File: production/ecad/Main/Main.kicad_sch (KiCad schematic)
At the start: 1 part, among them J1 61204021621

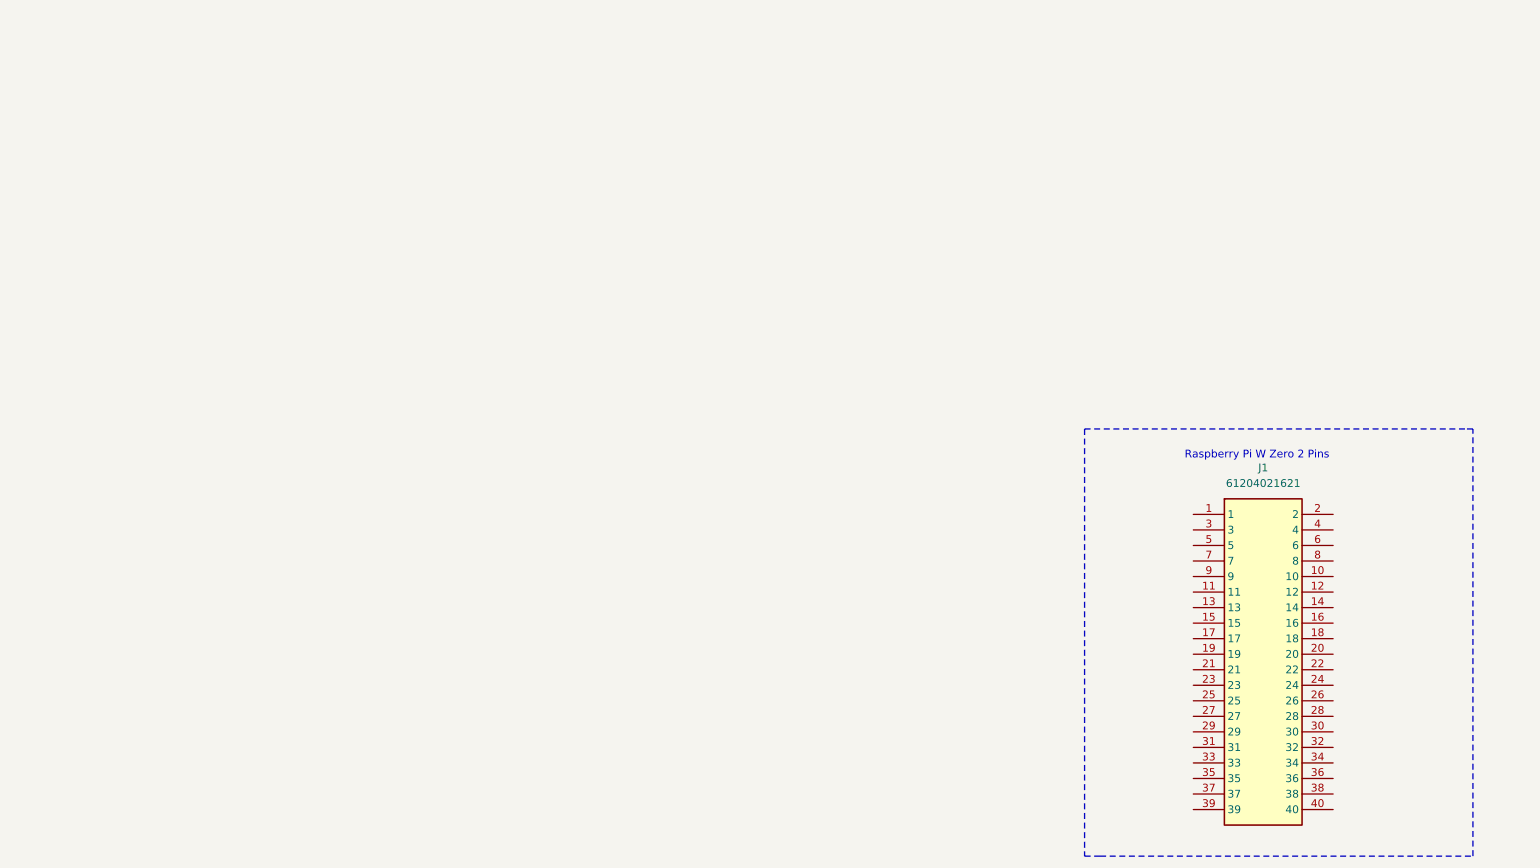
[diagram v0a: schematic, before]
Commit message: touches to schem
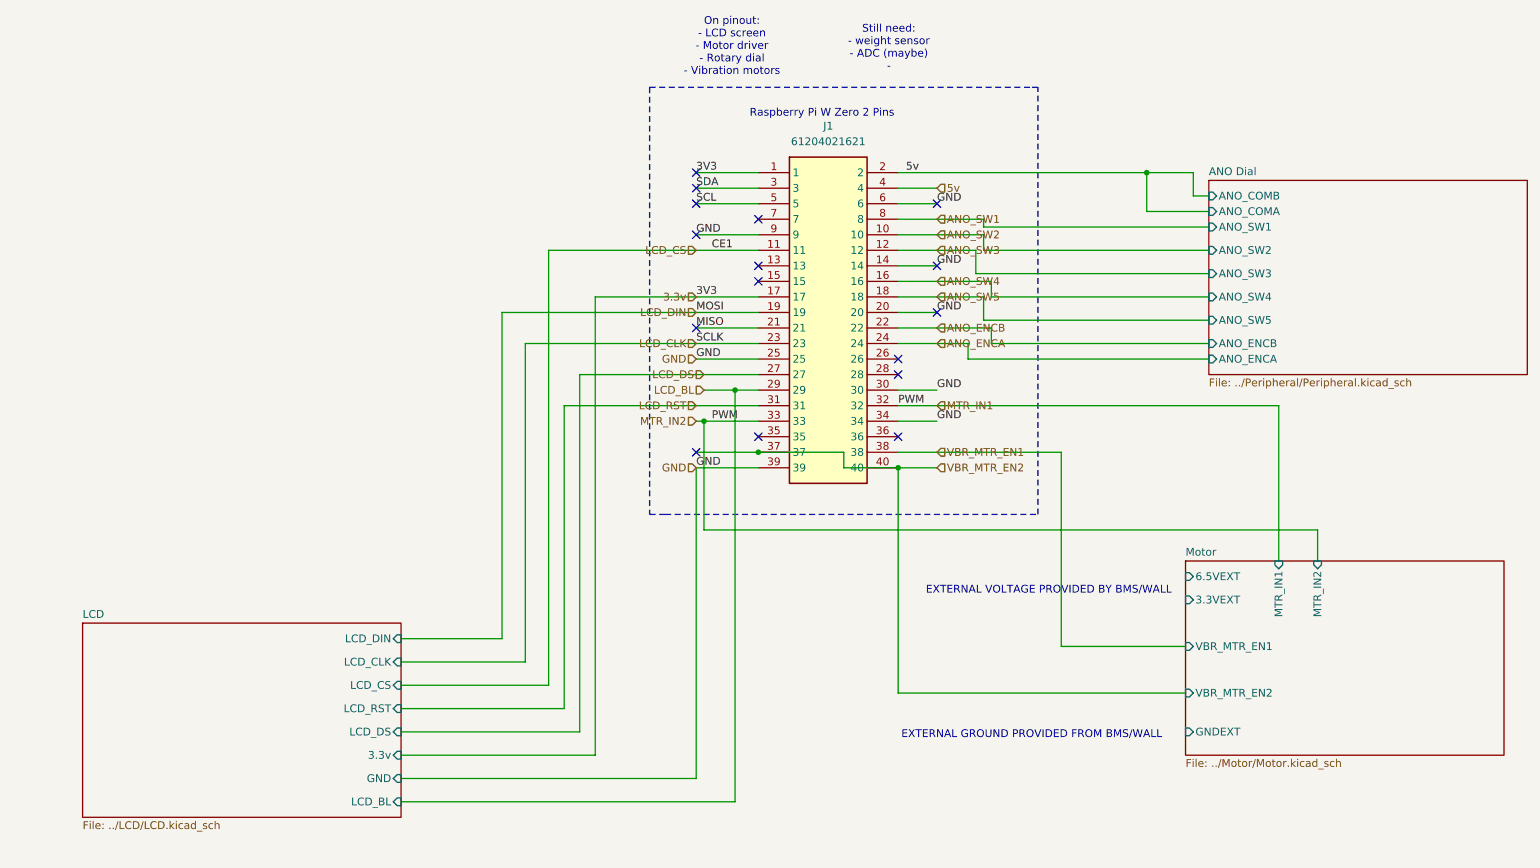
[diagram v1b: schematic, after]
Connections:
- net 3.3v: now reaches J1.1
- net 3.3v: now also J1.17
- net ANO_SW2: now reaches J1.10
- net LCD_CS: now reaches J1.11
- net ANO_SW3: now reaches J1.12
- net GND: now reaches J1.14
- net GND: now also J1.20, J1.25, J1.30, J1.34, J1.39, J1.6, J1.9
- net ANO_SW4: now reaches J1.16
- net ANO_SW5: now reaches J1.18
- net LCD_DIN: now reaches J1.19
- net 5v: now reaches J1.2
- net 5v: now also J1.4
- net MISO: now reaches J1.21
- net ANO_ENCB: now reaches J1.22
- net LCD_CLK: now reaches J1.23
- net ANO_ENCA: now reaches J1.24
- net LCD_DS: now reaches J1.27
- net LCD_BL: now reaches J1.29
- net SDA: now reaches J1.3
- net LCD_RST: now reaches J1.31
- net MTR_IN1: now reaches J1.32
- net MTR_IN1: now also J1.33
- net VBR_MTR_EN2: now reaches J1.37
- net VBR_MTR_EN2: now also J1.40
- net VBR_MTR_EN1: now reaches J1.38
- net SCL: now reaches J1.5
- net ANO_SW1: now reaches J1.8
- no-connect marks 0 -> 16
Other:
- added sheet ANO Dial (../Peripheral/Peripheral.kicad_sch)
- added sheet LCD (../LCD/LCD.kicad_sch)
- added sheet Motor (../Motor/Motor.kicad_sch)
- note added: "EXTERNAL GROUND PROVIDED FROM BMS/WALL"
- note added: "EXTERNAL VOLTAGE PROVIDED BY BMS/WALL"
- note added: "On pinout: - LCD screen - Motor driver - Rotary dial - Vibration motors"
- note added: "Still need: - weight sensor - ADC (maybe) -"
- moved on the sheet: J1

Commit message: schematic draft merged w neha
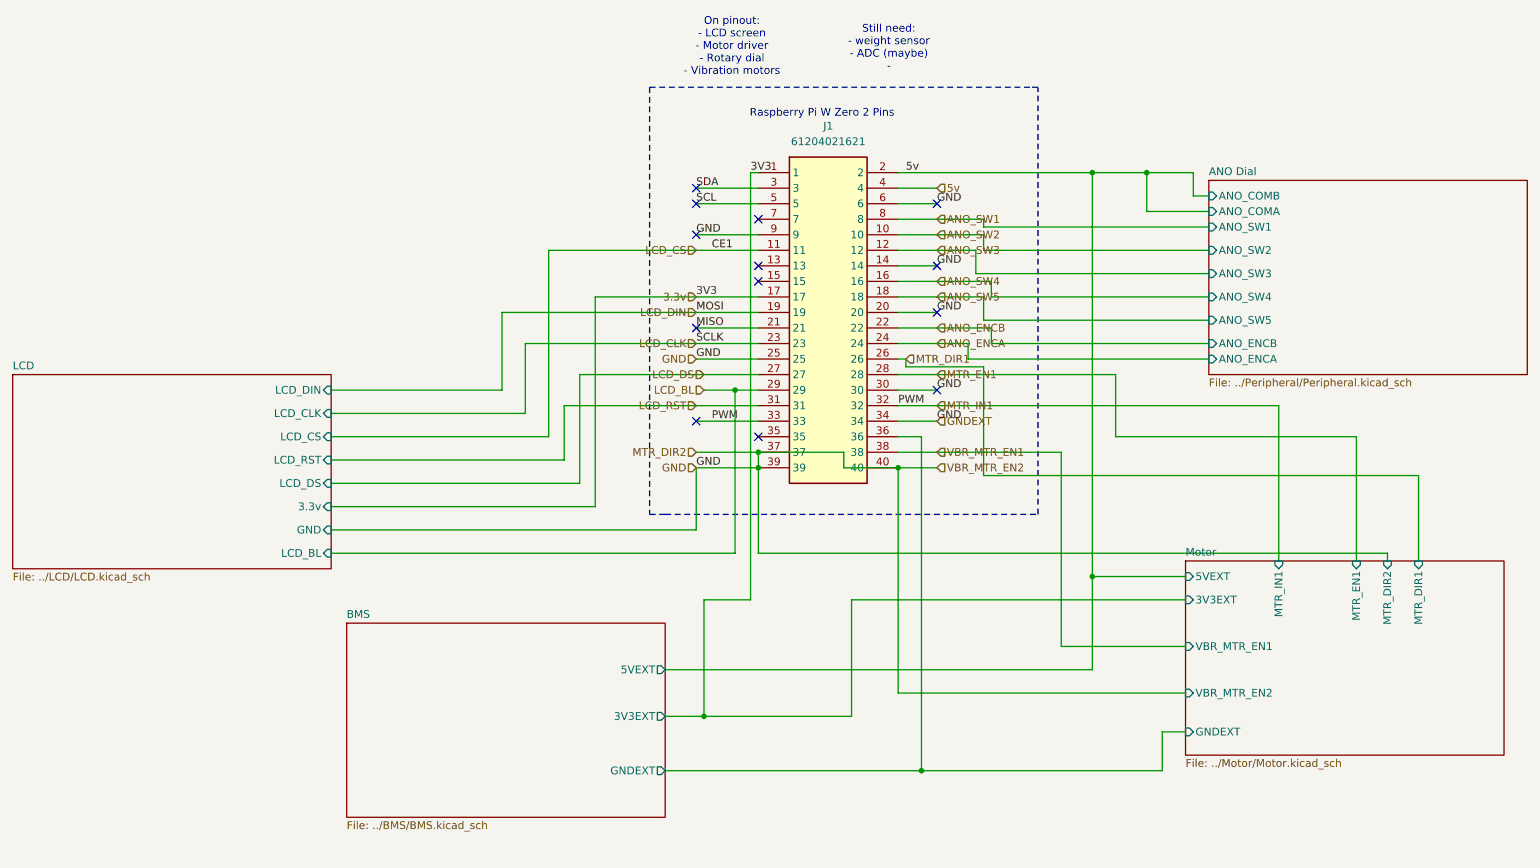
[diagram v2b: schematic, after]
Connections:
- net VBR_MTR_EN2 is gone; now on net GND: J1.37, J1.40
- net MTR_DIR1: now reaches J1.26
- net MTR_EN1: now reaches J1.28
- net BMS/GNDEXT: now reaches J1.36
- no-connect marks 16 -> 13
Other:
- added sheet BMS (../BMS/BMS.kicad_sch)
- sheet Motor ports: added 3V3EXT, 5VEXT, MTR_DIR1, MTR_DIR2, MTR_EN1; removed 3.3VEXT, 6.5VEXT, MTR_IN2
- note removed: "EXTERNAL GROUND PROVIDED FROM BMS/WALL"
- note removed: "EXTERNAL VOLTAGE PROVIDED BY BMS/WALL"

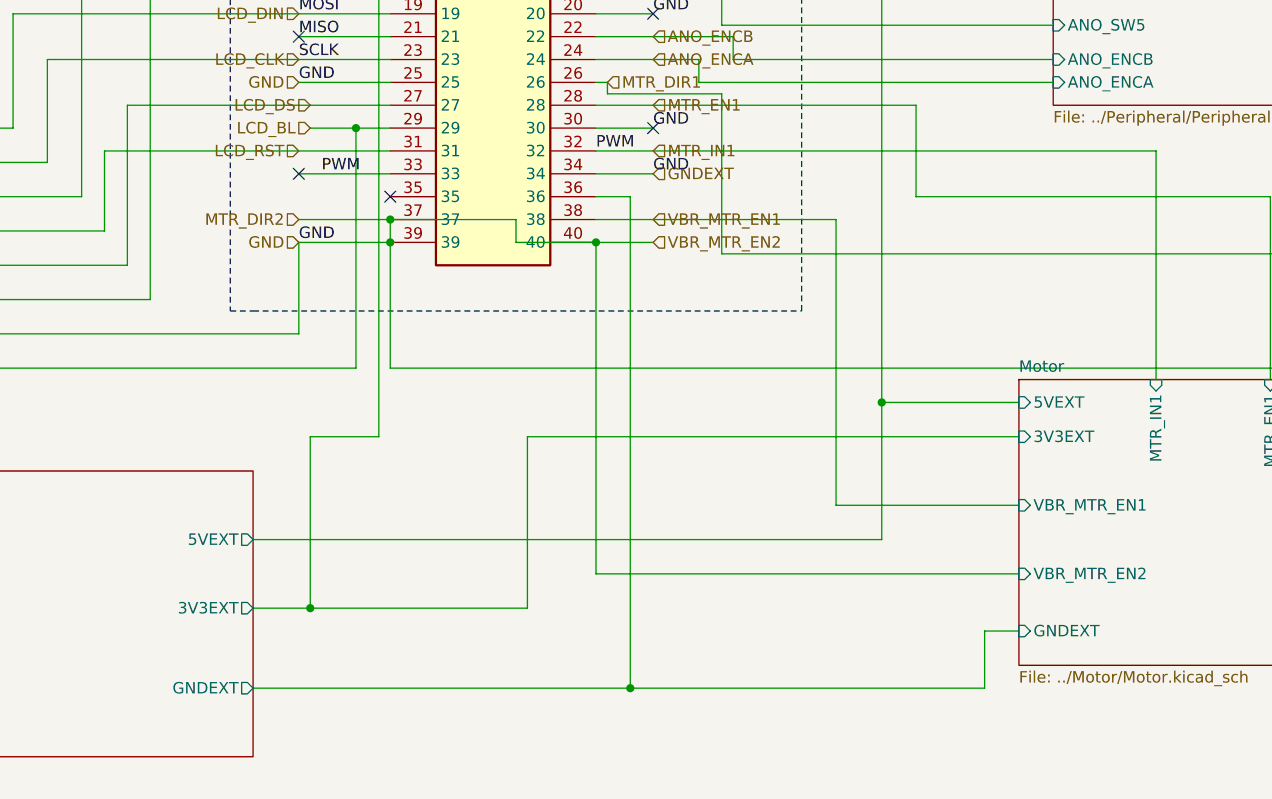
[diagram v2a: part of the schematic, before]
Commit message: feedback from Billayyy
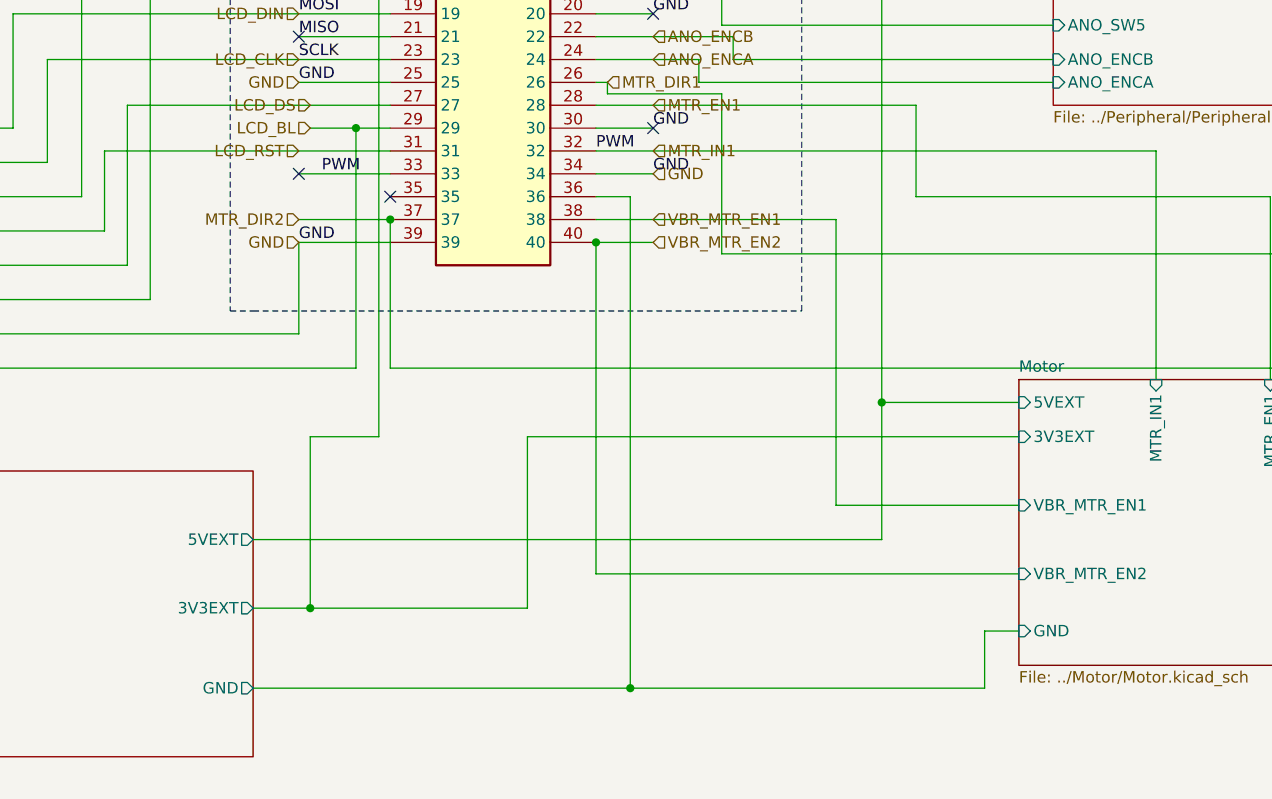
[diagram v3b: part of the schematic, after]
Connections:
- net GND: no longer J1.37, J1.40
- net BMS/GNDEXT renamed BMS/GND
- new net MTR_DIR2: J1.37
- new net VBR_MTR_EN2: J1.40
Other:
- sheet BMS ports: added GND; removed GNDEXT
- sheet Motor ports: added GND; removed GNDEXT
